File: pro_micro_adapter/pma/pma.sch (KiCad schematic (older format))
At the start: 4 parts, among them J1 Lily58-cache_MJ-4PP-9, J2 4PIN, J3 4PIN, U1 ProMicro

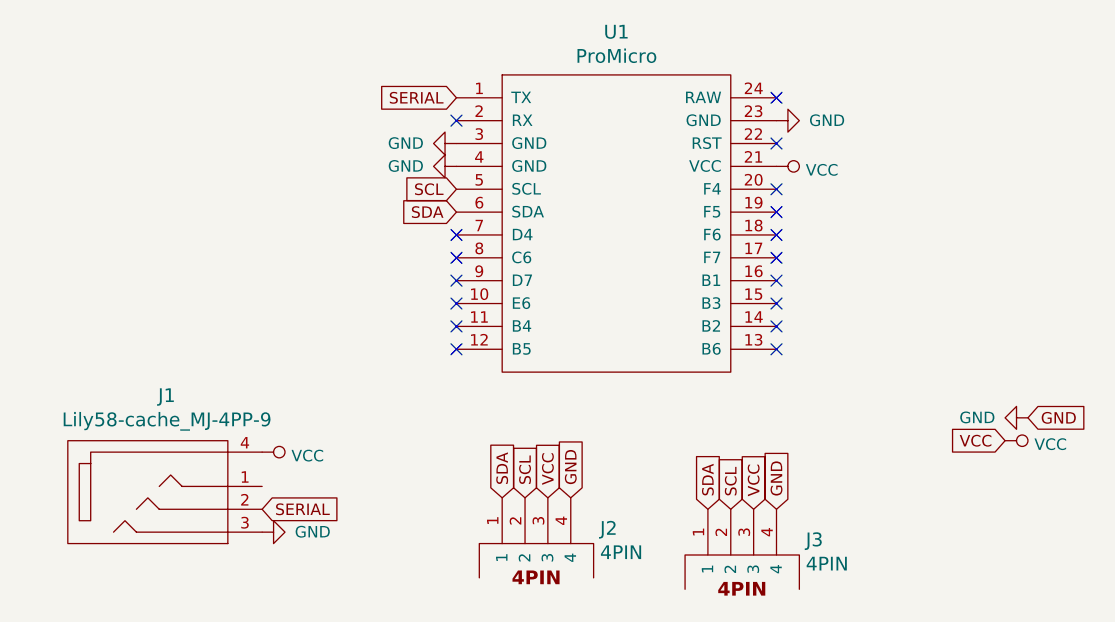
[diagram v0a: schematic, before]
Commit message: silk
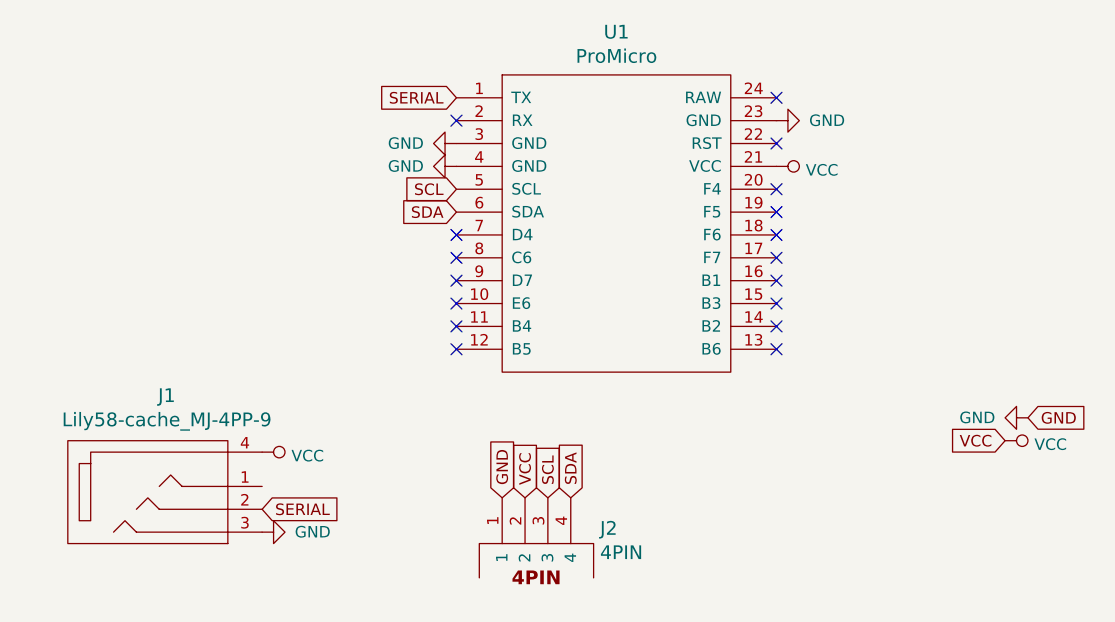
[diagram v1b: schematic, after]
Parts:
- removed J3: 4PIN, Connector_PinHeader_2.54mm:PinHeader_1x04_P2.54mm_Vertical, symbol 4pin:4PIN
- J1: footprint Custom Footies:PJ-606-6A -> Lily58-footprint:MJ-4PP-9
- J2: footprint Connector_PinHeader_2.54mm:PinHeader_1x04_P2.54mm_Vertical -> Custom Footies:PinHeader_1x04_P2.54mm_REVERSIBLE
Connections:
- net GND: now also J2.1; no longer J2.4
- net SCL: now also J2.3; no longer J2.2
- net SDA: now also J2.4; no longer J2.1
- net VCC: now also J2.2; no longer J2.3
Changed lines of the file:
@@
 EESchema Schematic File Version 4
+LIBS:pma-cache
 EELAYER 30 0
 EELAYER END
@@
 F 0 "J1" H 5733 3997 60  0000 C CNN
 F 1 "Lily58-cache_MJ-4PP-9" H 5733 3891 60  0000 C CNN
-F 2 "Custom Footies:PJ-606-6A" H 5700 3600 60  0001 C CNN
+F 2 "Lily58-footprint:MJ-4PP-9" H 5700 3600 60  0001 C CNN
 F 3 "" H 5700 3600 60  0000 C CNN
 	1    5700 3600
@@
 F 0 "J2" V 7466 3622 60  0000 R CNN
 F 1 "4PIN" V 7360 3622 60  0000 R CNN
-F 2 "Connector_PinHeader_2.54mm:PinHeader_1x04_P2.54mm_Vertical" H 7400 3850 60  0001 C CNN
+F 2 "Custom Footies:PinHeader_1x04_P2.54mm_REVERSIBLE" H 7400 3850 60  0001 C CNN
 F 3 "" H 7400 3850 60  0000 C CNN
 	1    7350 3900
 	0    -1   -1   0
 $EndComp
+Text GLabel 7500 3650 1    50   Input ~ 0
+SDA
+Text GLabel 7400 3650 1    50   Input ~ 0
+SCL
+Text GLabel 7300 3650 1    50   Input ~ 0
+VCC
 Text GLabel 7200 3650 1    50   Input ~ 0
-SDA
-Text GLabel 7300 3650 1    50   Input ~ 0
-SCL
-Text GLabel 7400 3650 1    50   Input ~ 0
-VCC
-Text GLabel 7500 3650 1    50   Input ~ 0
 GND
 Text GLabel 9500 3300 2    50   Input ~ 0
@@
 	0    1    1    0
 $EndComp
-$Comp
-L 4pin:4PIN J3
-U 1 1 60DD2E48
-P 8250 3950
-F 0 "J3" V 8366 3672 60  0000 R CNN
-F 1 "4PIN" V 8260 3672 60  0000 R CNN
-F 2 "Connector_PinHeader_2.54mm:PinHeader_1x04_P2.54mm_Vertical" H 8300 3900 60  0001 C CNN
-F 3 "" H 8300 3900 60  0000 C CNN
-	1    8250 3950
-	0    -1   -1   0
-$EndComp
-Text GLabel 8100 3700 1    50   Input ~ 0
-SDA
-Text GLabel 8200 3700 1    50   Input ~ 0
-SCL
-Text GLabel 8300 3700 1    50   Input ~ 0
-VCC
-Text GLabel 8400 3700 1    50   Input ~ 0
-GND
 $EndSCHEMATC
